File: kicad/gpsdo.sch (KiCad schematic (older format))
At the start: 45 parts, among them J1 Conn_Coaxial, J2 Conn_01x04_Male, J3 Conn_01x04_Male, J4 Conn_01x04_Male, J5 Conn_01x04_Male, J6 Conn_01x04_Male, U1 MSP430F5171IDA, U10 74AUC1G79, U11 47L64, U2 MAX-8Q, U3 549CAAC000111BBG, U4 Si7051-A20, U6 74LVC1G08, U7 74LVC1G08, U8 74AUC1G79, U9 74LVC1G86

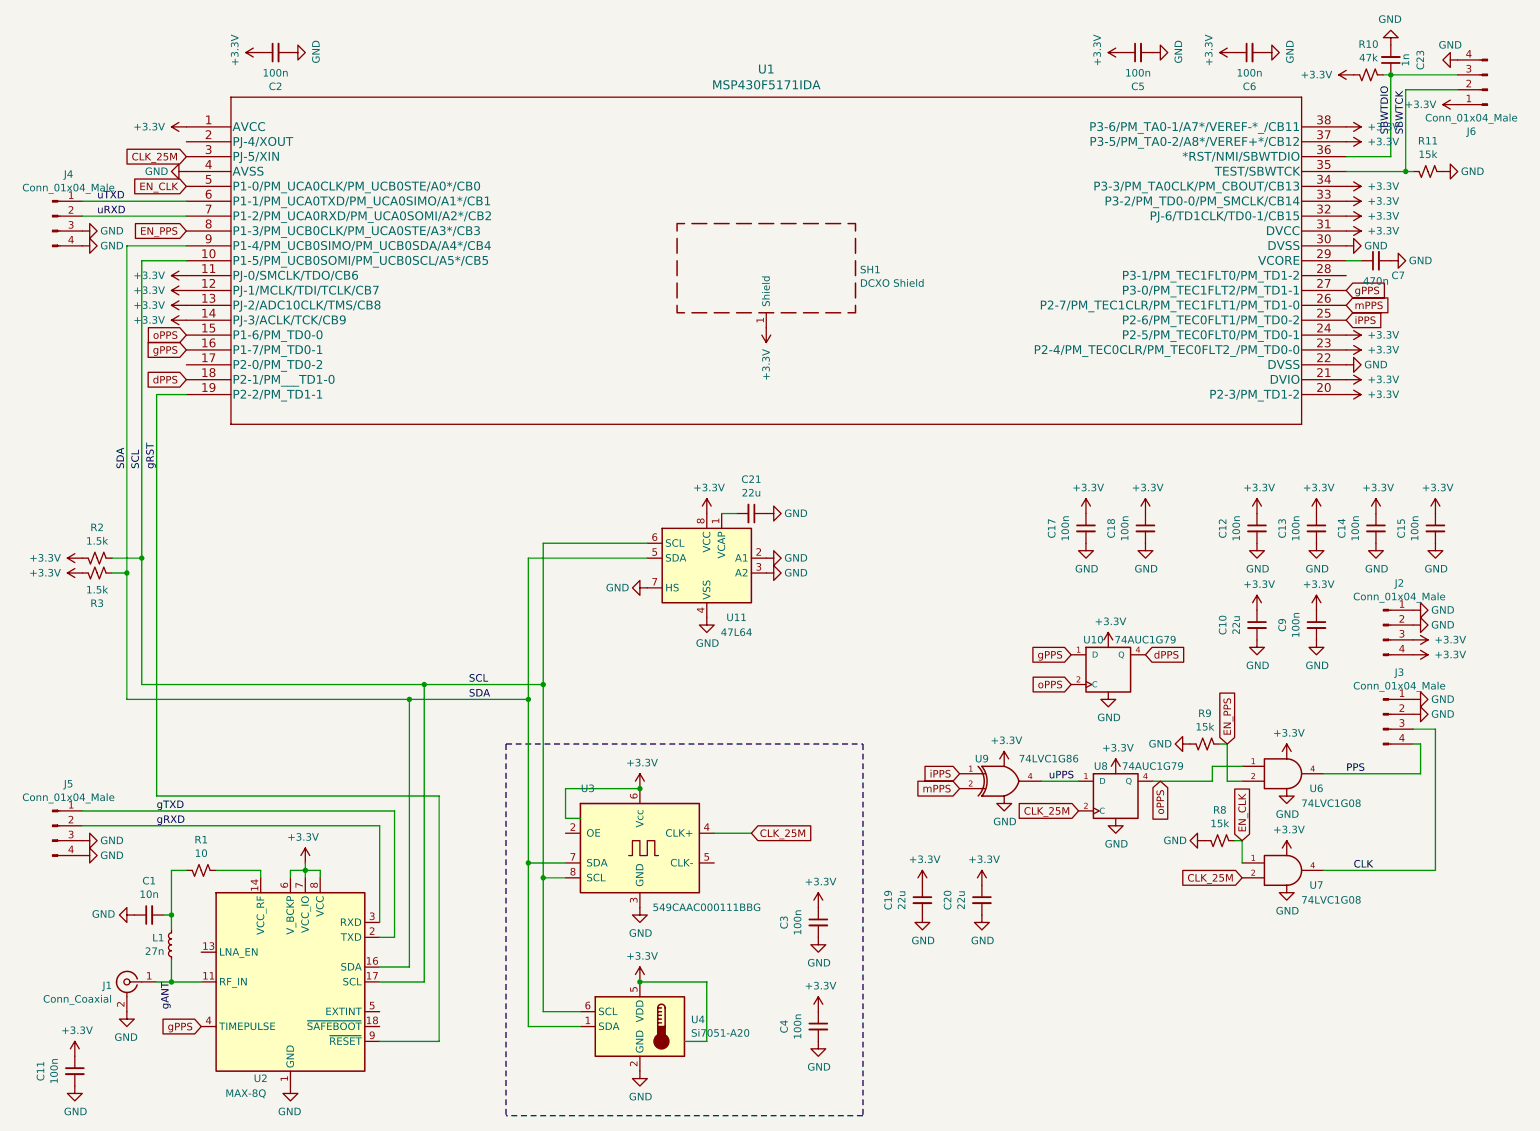
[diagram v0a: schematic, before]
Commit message: update pcb layout
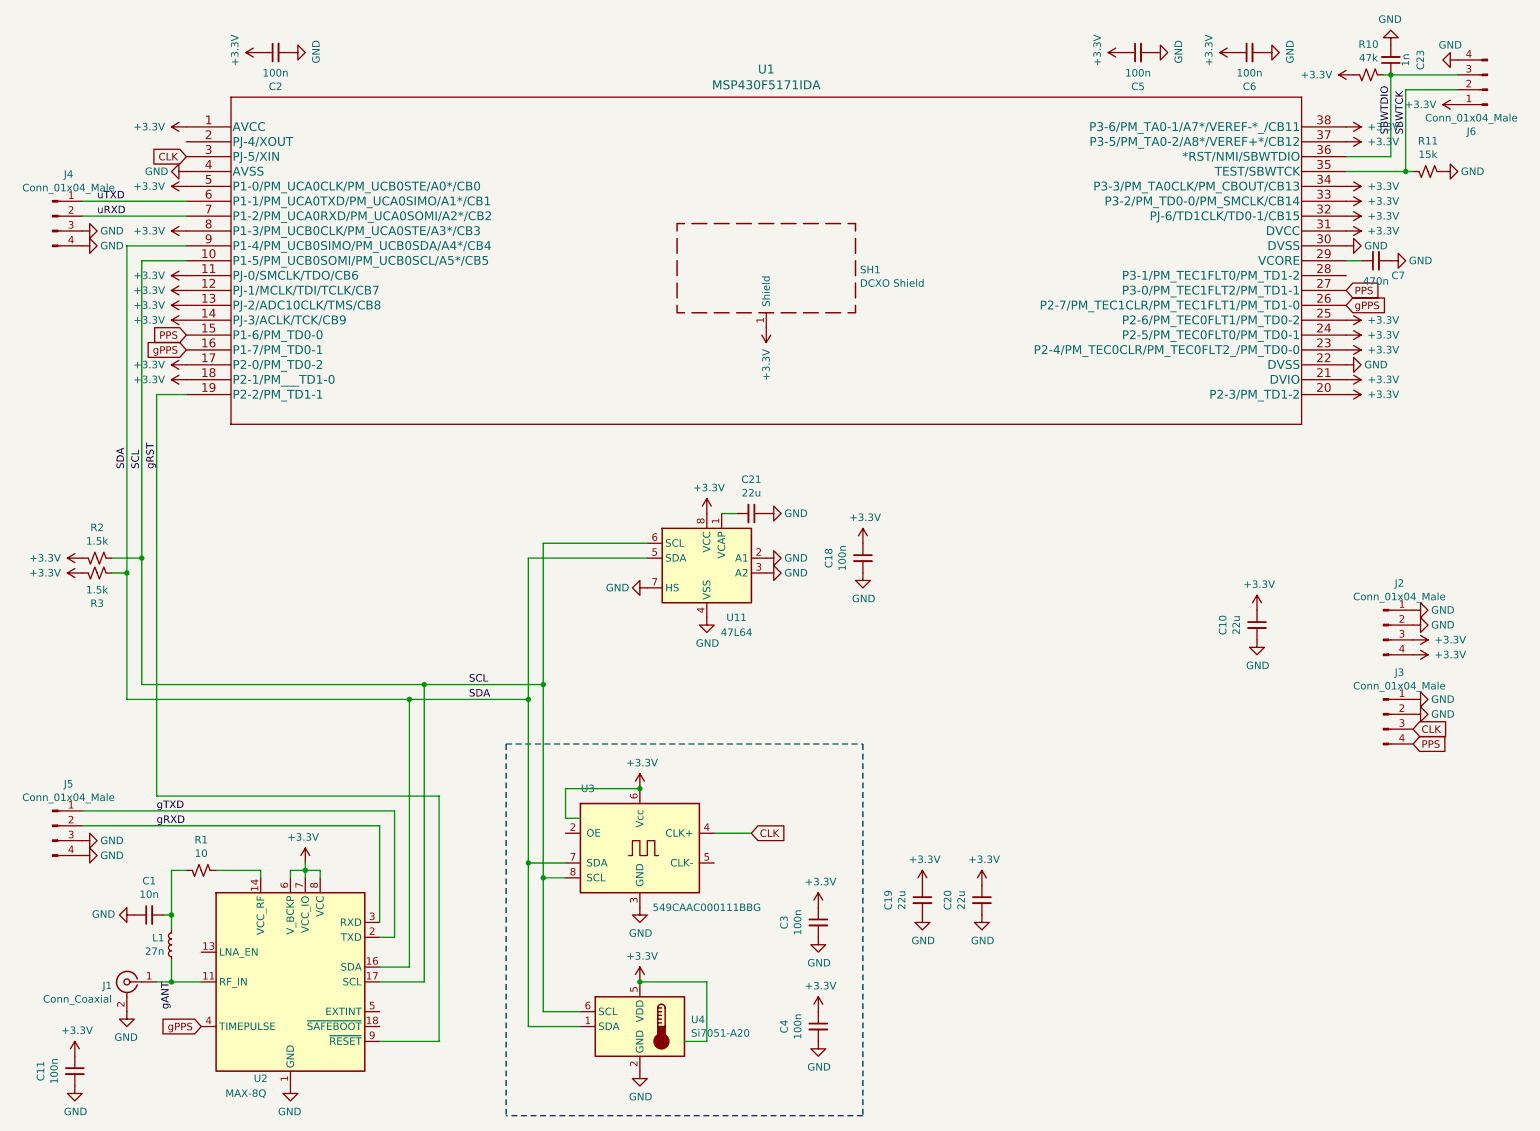
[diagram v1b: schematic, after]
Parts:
- removed C12, C13, C14, C15, C17, C9: 100n, Resistor_SMD:R_0603_1608Metric, symbol Device:C_Small
- removed R8, R9: 15k, Resistor_SMD:R_0603_1608Metric, symbol Device:R_Small_US
- removed U10, U8: 74AUC1G79, Package_TO_SOT_SMD:SOT-23-5, symbol 74xGxx:74AUC1G79
- removed U6, U7: 74LVC1G08, Package_TO_SOT_SMD:SOT-23-5, symbol 74xGxx:74LVC1G08
- removed U9: 74LVC1G86, Package_TO_SOT_SMD:SOT-23-5, symbol 74xGxx:74LVC1G86
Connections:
- net CLK_25M is gone; now on net CLK: U1.3 (PJ-5/XIN), U3.4 (CLK+)
- net EN_CLK is gone; now on net +3V3: U1.5 (P1-0/PM_UCA0CLK/PM_UCB0STE/A0*/CB0)
- net EN_PPS is gone; now on net +3V3: U1.8 (P1-3/PM_UCB0CLK/PM_UCA0STE/A3*/CB3)
- net dPPS is gone; now on net +3V3: U1.18 (P2-1/PM___TD1-0)
- net iPPS is gone; now on net +3V3: U1.25 (P2-6/PM_TEC0FLT1/PM_TD0-2)
- net mPPS is gone; now on net gPPS: U1.26 (P2-7/PM_TEC1CLR/PM_TEC1FLT1/PM_TD1-0)
- net oPPS is gone; now on net PPS: U1.15 (P1-6/PM_TD0-0)
- net +3V3: now also U1.17 (P2-0/PM_TD0-2)
- net PPS: now also U1.27 (P3-0/PM_TEC1FLT2/PM_TD1-1)
- net gPPS: no longer U1.27 (P3-0/PM_TEC1FLT2/PM_TD1-1)
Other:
- moved on the sheet: C18

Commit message: update pcb layout
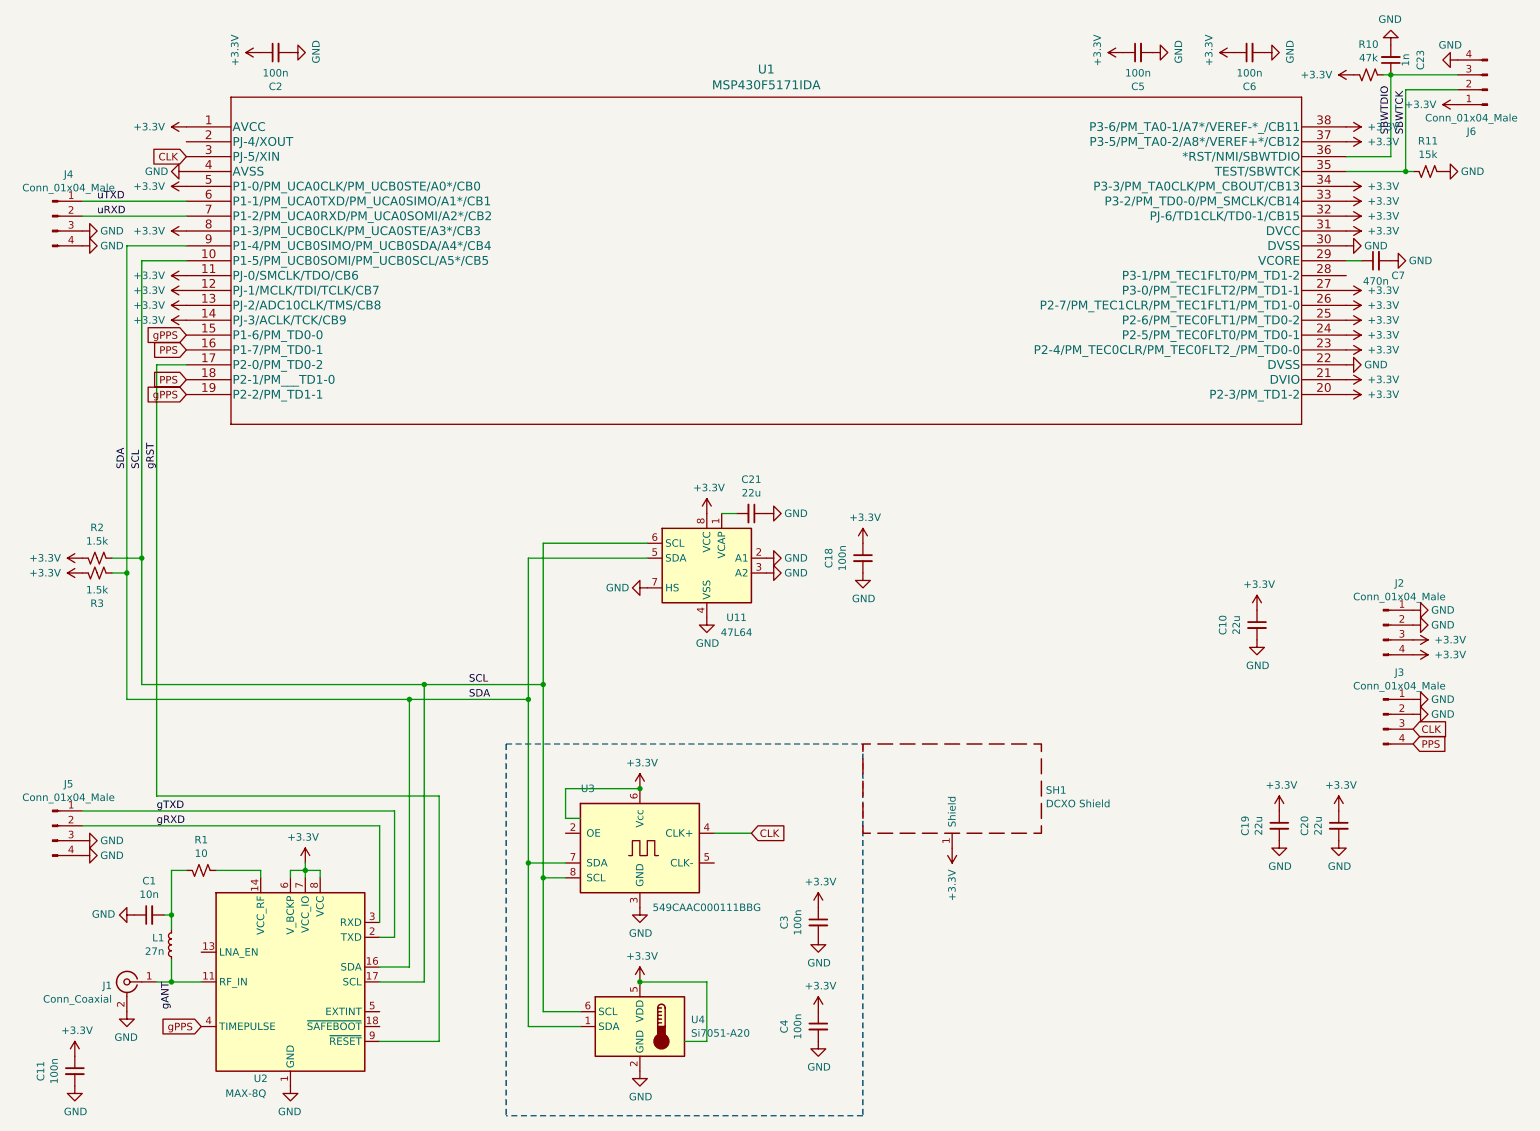
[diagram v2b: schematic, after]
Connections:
- net +3V3: now also U1.26 (P2-7/PM_TEC1CLR/PM_TEC1FLT1/PM_TD1-0), U1.27 (P3-0/PM_TEC1FLT2/PM_TD1-1); no longer U1.17 (P2-0/PM_TD0-2), U1.18 (P2-1/PM___TD1-0)
- net PPS: now also U1.16 (P1-7/PM_TD0-1), U1.18 (P2-1/PM___TD1-0); no longer U1.15 (P1-6/PM_TD0-0), U1.27 (P3-0/PM_TEC1FLT2/PM_TD1-1)
- net gPPS: now also U1.15 (P1-6/PM_TD0-0), U1.19 (P2-2/PM_TD1-1); no longer U1.16 (P1-7/PM_TD0-1), U1.26 (P2-7/PM_TEC1CLR/PM_TEC1FLT1/PM_TD1-0)
- net gRST: now also U1.17 (P2-0/PM_TD0-2); no longer U1.19 (P2-2/PM_TD1-1)
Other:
- moved on the sheet: C19, C20, SH1
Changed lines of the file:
@@
 Text GLabel 1700 7250 0    50   Input ~ 0
 gPPS
-Text GLabel 1600 2700 0    50   Input ~ 0
+Text GLabel 1600 3000 0    50   Input ~ 0
 gPPS
 $Comp
@@
 	0    -1   -1   0
 $EndComp
-Text GLabel 1600 2600 0    50   Input ~ 0
+Text GLabel 1600 2900 0    50   Input ~ 0
 PPS
 Wire Wire Line
@@
 Wire Wire Line
 	3300 5700 1400 5700
-Wire Wire Line
-	1400 5700 1400 3000
-Wire Wire Line
-	1400 3000 1600 3000
 $Comp
 L Device:C_Small C11
@@
 	1    0    0    -1
 $EndComp
-Text GLabel 9400 2300 2    50   Input ~ 0
+Text GLabel 1600 2700 0    50   Input ~ 0
 PPS
 $Comp
@@
 	0    1    -1   0
 $EndComp
-Text GLabel 9400 2400 2    50   Input ~ 0
+Text GLabel 1600 2600 0    50   Input ~ 0
 gPPS
 $Comp
@@
 L Device:C_Small C19
 U 1 1 61093E5D
-P 6550 6400
-F 0 "C19" V 6321 6400 50  0000 C CNN
-F 1 "22u" V 6412 6400 50  0000 C CNN
-F 2 "Capacitor_SMD:C_0805_2012Metric" H 6550 6400 50  0001 C CNN
-F 3 "~" H 6550 6400 50  0001 C CNN
-	1    6550 6400
+P 8950 5900
+F 0 "C19" V 8721 5900 50  0000 C CNN
+F 1 "22u" V 8812 5900 50  0000 C CNN
+F 2 "Capacitor_SMD:C_0805_2012Metric" H 8950 5900 50  0001 C CNN
+F 3 "~" H 8950 5900 50  0001 C CNN
+	1    8950 5900
 	1    0    0    -1
 $EndComp
@@
 L power:GND #PWR0171
 U 1 1 61093E63
-P 6550 6500
-F 0 "#PWR0171" H 6550 6250 50  0001 C CNN
-F 1 "GND" H 6555 6327 50  0000 C CNN
-F 2 "" H 6550 6500 50  0001 C CNN
-F 3 "" H 6550 6500 50  0001 C CNN
-	1    6550 6500
+P 8950 6000
+F 0 "#PWR0171" H 8950 5750 50  0001 C CNN
+F 1 "GND" H 8955 5827 50  0000 C CNN
+F 2 "" H 8950 6000 50  0001 C CNN
+F 3 "" H 8950 6000 50  0001 C CNN
+	1    8950 6000
 	1    0    0    -1
 $EndComp
@@
 L power:+3.3V #PWR0172
 U 1 1 61093E69
-P 6550 6300
-F 0 "#PWR0172" H 6550 6150 50  0001 C CNN
-F 1 "+3.3V" H 6565 6473 50  0000 C CNN
-F 2 "" H 6550 6300 50  0001 C CNN
-F 3 "" H 6550 6300 50  0001 C CNN
-	1    6550 6300
+P 8950 5800
+F 0 "#PWR0172" H 8950 5650 50  0001 C CNN
+F 1 "+3.3V" H 8965 5973 50  0000 C CNN
+F 2 "" H 8950 5800 50  0001 C CNN
+F 3 "" H 8950 5800 50  0001 C CNN
+	1    8950 5800
 	1    0    0    -1
 $EndComp
@@
 L Device:C_Small C20
 U 1 1 61097B5B
-P 6950 6400
-F 0 "C20" V 6721 6400 50  0000 C CNN
-F 1 "22u" V 6812 6400 50  0000 C CNN
-F 2 "Capacitor_SMD:C_0805_2012Metric" H 6950 6400 50  0001 C CNN
-F 3 "~" H 6950 6400 50  0001 C CNN
-	1    6950 6400
+P 9350 5900
+F 0 "C20" V 9121 5900 50  0000 C CNN
+F 1 "22u" V 9212 5900 50  0000 C CNN
+F 2 "Capacitor_SMD:C_0805_2012Metric" H 9350 5900 50  0001 C CNN
+F 3 "~" H 9350 5900 50  0001 C CNN
+	1    9350 5900
 	1    0    0    -1
 $EndComp
@@
 L power:GND #PWR0173
 U 1 1 61097B61
-P 6950 6500
-F 0 "#PWR0173" H 6950 6250 50  0001 C CNN
-F 1 "GND" H 6955 6327 50  0000 C CNN
-F 2 "" H 6950 6500 50  0001 C CNN
-F 3 "" H 6950 6500 50  0001 C CNN
-	1    6950 6500
+P 9350 6000
+F 0 "#PWR0173" H 9350 5750 50  0001 C CNN
+F 1 "GND" H 9355 5827 50  0000 C CNN
+F 2 "" H 9350 6000 50  0001 C CNN
+F 3 "" H 9350 6000 50  0001 C CNN
+	1    9350 6000
 	1    0    0    -1
 $EndComp
@@
 L power:+3.3V #PWR0174
 U 1 1 61097B67
-P 6950 6300
-F 0 "#PWR0174" H 6950 6150 50  0001 C CNN
-F 1 "+3.3V" H 6965 6473 50  0000 C CNN
-F 2 "" H 6950 6300 50  0001 C CNN
-F 3 "" H 6950 6300 50  0001 C CNN
-	1    6950 6300
+P 9350 5800
+F 0 "#PWR0174" H 9350 5650 50  0001 C CNN
+F 1 "+3.3V" H 9365 5973 50  0000 C CNN
+F 2 "" H 9350 5800 50  0001 C CNN
+F 3 "" H 9350 5800 50  0001 C CNN
+	1    9350 5800
 	1    0    0    -1
 $EndComp
@@
 L Device:RF_Shield_One_Piece SH1
 U 1 1 610DBF58
-P 5500 2150
-F 0 "SH1" H 6130 2139 50  0000 L CNN
-F 1 "DCXO Shield" H 6130 2048 50  0000 L CNN
-F 2 "RF_Shielding:Laird_Technologies_BMI-S-102_16.50x16.50mm" H 5500 2050 50  0001 C CNN
-F 3 "~" H 5500 2050 50  0001 C CNN
-	1    5500 2150
+P 6750 5650
+F 0 "SH1" H 7380 5639 50  0000 L CNN
+F 1 "DCXO Shield" H 7380 5548 50  0000 L CNN
+F 2 "RF_Shielding:Laird_Technologies_BMI-S-102_16.50x16.50mm" H 6750 5550 50  0001 C CNN
+F 3 "~" H 6750 5550 50  0001 C CNN
+	1    6750 5650
 	1    0    0    -1
 $EndComp
@@
 L power:+3.3V #PWR0177
 U 1 1 610E291C
-P 5500 2550
-F 0 "#PWR0177" H 5500 2400 50  0001 C CNN
-F 1 "+3.3V" V 5500 2800 50  0000 C CNN
-F 2 "" H 5500 2550 50  0001 C CNN
-F 3 "" H 5500 2550 50  0001 C CNN
-	1    5500 2550
+P 6750 6050
+F 0 "#PWR0177" H 6750 5900 50  0001 C CNN
+F 1 "+3.3V" V 6750 6300 50  0000 C CNN
+F 2 "" H 6750 6050 50  0001 C CNN
+F 3 "" H 6750 6050 50  0001 C CNN
+	1    6750 6050
 	-1   0    0    1
 $EndComp
@@
 $EndComp
 $Comp
-L power:+3.3V #PWR0140
-U 1 1 61108A0C
-P 1600 2900
-F 0 "#PWR0140" H 1600 2750 50  0001 C CNN
-F 1 "+3.3V" V 1600 3150 50  0000 C CNN
-F 2 "" H 1600 2900 50  0001 C CNN
-F 3 "" H 1600 2900 50  0001 C CNN
-	1    1600 2900
-	0    -1   -1   0
-$EndComp
-$Comp
-L power:+3.3V #PWR0121
-U 1 1 611086AF
-P 1600 2800
-F 0 "#PWR0121" H 1600 2650 50  0001 C CNN
-F 1 "+3.3V" V 1600 3050 50  0000 C CNN
-F 2 "" H 1600 2800 50  0001 C CNN
-F 3 "" H 1600 2800 50  0001 C CNN
-	1    1600 2800
-	0    -1   -1   0
-$EndComp
-$Comp
 L power:+3.3V #PWR0122
 U 1 1 610D583A
@@
 CLK
 $Comp
-L power:+3.3V #PWR?
+L power:+3.3V #PWR0114
 U 1 1 611DA105
 P 1600 1900
-F 0 "#PWR?" H 1600 1750 50  0001 C CNN
+F 0 "#PWR0114" H 1600 1750 50  0001 C CNN
 F 1 "+3.3V" V 1600 2150 50  0000 C CNN
 F 2 "" H 1600 1900 50  0001 C CNN
@@
 $EndComp
 $Comp
-L power:+3.3V #PWR?
+L power:+3.3V #PWR0121
 U 1 1 611DA46C
 P 1600 1600
-F 0 "#PWR?" H 1600 1450 50  0001 C CNN
+F 0 "#PWR0121" H 1600 1450 50  0001 C CNN
 F 1 "+3.3V" V 1600 1850 50  0000 C CNN
 F 2 "" H 1600 1600 50  0001 C CNN
@@
 	0    -1   -1   0
 $EndComp
+Wire Wire Line
+	1400 5700 1400 2800
+Wire Wire Line
+	1400 2800 1600 2800
+$Comp
+L power:+3.3V #PWR0132
+U 1 1 61108331
+P 9400 2400
+F 0 "#PWR0132" H 9400 2250 50  0001 C CNN
+F 1 "+3.3V" V 9400 2650 50  0000 C CNN
+F 2 "" H 9400 2400 50  0001 C CNN
+F 3 "" H 9400 2400 50  0001 C CNN
+	1    9400 2400
+	0    1    1    0
+$EndComp
+$Comp
+L power:+3.3V #PWR0133
+U 1 1 611085DD
+P 9400 2300
+F 0 "#PWR0133" H 9400 2150 50  0001 C CNN
+F 1 "+3.3V" V 9400 2550 50  0000 C CNN
+F 2 "" H 9400 2300 50  0001 C CNN
+F 3 "" H 9400 2300 50  0001 C CNN
+	1    9400 2300
+	0    1    1    0
+$EndComp
 $EndSCHEMATC
